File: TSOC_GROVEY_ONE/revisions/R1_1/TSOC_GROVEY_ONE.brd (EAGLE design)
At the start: 44.5 x 30.5 mm, 53 parts, among them J3 NO, J4 6p-2.54, U1 MIC5219 3.3V, U2 ATMEGA328, X1 16MHZ

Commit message: update to Rev 2.0
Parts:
- R10, R4, R5, R7, R8, R9: value 1K 1/10W -> 1K
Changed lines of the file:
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@@
 <setting verticaltext="up"/>
 </settings>
-<grid distance="10" unitdist="mil" unit="mil" style="lines" multiple="1" display="yes" altdistance="5" altunitdist="mil" altunit="mil"/>
+<grid distance="10" unitdist="mil" unit="mm" style="lines" multiple="1" display="yes" altdistance="5" altunitdist="mil" altunit="mil"/>
 <layers>
 <layer number="1" name="Top" color="4" fill="1" visible="yes" active="yes"/>
@@
 <layer number="23" name="tOrigins" color="15" fill="1" visible="yes" active="yes"/>
 <layer number="24" name="bOrigins" color="15" fill="1" visible="yes" active="yes"/>
-<layer number="25" name="tNames" color="7" fill="1" visible="no" active="yes"/>
+<layer number="25" name="tNames" color="7" fill="1" visible="yes" active="yes"/>
 <layer number="26" name="bNames" color="7" fill="1" visible="yes" active="yes"/>
 <layer number="27" name="tValues" color="7" fill="1" visible="no" active="yes"/>
@@
 <layer number="220" name="220bmp" color="21" fill="1" visible="no" active="no"/>
 <layer number="221" name="221bmp" color="22" fill="1" visible="no" active="no"/>
-<layer number="222" name="222bmp" color="23" fill="1" visible="no" active="no"/>
 <layer number="223" name="223bmp" color="24" fill="1" visible="no" active="no"/>
 <layer number="224" name="224bmp" color="25" fill="1" visible="no" active="no"/>
@@
 <attribute name="VALUE" x="42.926" y="24.257" size="0.889" layer="27" font="vector" ratio="11" rot="R270"/>
 </element>
-<element name="R9" library="Seeed-Resistor-2016" package="R0603" value="1K 1/10W" x="34.29" y="20.574" smashed="yes">
+<element name="R9" library="Seeed-Resistor-2016" package="R0603" value="1K" x="34.29" y="20.574" smashed="yes">
 <attribute name="NAME" x="33.528" y="19.939" size="0.8128" layer="25" font="vector" ratio="15" rot="R90"/>
-<attribute name="VALUE" value="1K 1/10W" x="33.274" y="19.431" size="0.4064" layer="27" font="vector"/>
-<attribute name="MPN" value="RC0603JR-071KL" x="34.29" y="20.574" size="1.778" layer="27" display="off"/>
-</element>
-<element name="R10" library="Seeed-Resistor-2016" package="R0603" value="1K 1/10W" x="34.29" y="23.622" smashed="yes" rot="R180">
+<attribute name="VALUE" value="2.2K" x="33.274" y="19.431" size="0.4064" layer="27" font="vector"/>
+<attribute name="MPN" value="RC0603JR-072K2L" x="34.29" y="20.574" size="1.778" layer="27" display="off"/>
+</element>
+<element name="R10" library="Seeed-Resistor-2016" package="R0603" value="1K" x="34.29" y="23.622" smashed="yes" rot="R180">
 <attribute name="NAME" x="32.766" y="24.257" size="0.8128" layer="25" font="vector" ratio="15" rot="R270"/>
-<attribute name="VALUE" value="1K 1/10W" x="35.306" y="24.765" size="0.4064" layer="27" font="vector" rot="R180"/>
-<attribute name="MPN" value="RC0603JR-071KL" x="34.29" y="23.622" size="1.778" layer="27" rot="R180" display="off"/>
-</element>
-<element name="R7" library="Seeed-Resistor-2016" package="R0603" value="1K 1/10W" x="34.29" y="10.16" smashed="yes">
+<attribute name="VALUE" value="2.2K" x="35.306" y="24.765" size="0.4064" layer="27" font="vector" rot="R180"/>
+<attribute name="MPN" value="RC0603JR-072K2L" x="34.29" y="23.622" size="1.778" layer="27" rot="R180" display="off"/>
+</element>
+<element name="R7" library="Seeed-Resistor-2016" package="R0603" value="1K" x="34.29" y="10.16" smashed="yes">
 <attribute name="NAME" x="33.528" y="9.525" size="0.8128" layer="25" font="vector" ratio="15" rot="R90"/>
-<attribute name="VALUE" value="1K 1/10W" x="33.274" y="9.017" size="0.4064" layer="27" font="vector"/>
-<attribute name="MPN" value="RC0603JR-071KL" x="34.29" y="10.16" size="1.778" layer="27" display="off"/>
-</element>
-<element name="R8" library="Seeed-Resistor-2016" package="R0603" value="1K 1/10W" x="34.29" y="13.208" smashed="yes" rot="R180">
+<attribute name="VALUE" value="2.2K" x="33.274" y="9.017" size="0.4064" layer="27" font="vector"/>
+<attribute name="MPN" value="RC0603JR-072K2L" x="34.29" y="10.16" size="1.778" layer="27" display="off"/>
+</element>
+<element name="R8" library="Seeed-Resistor-2016" package="R0603" value="1K" x="34.29" y="13.208" smashed="yes" rot="R180">
 <attribute name="NAME" x="33.528" y="12.573" size="0.8128" layer="25" font="vector" ratio="15" rot="R90"/>
-<attribute name="VALUE" value="1K 1/10W" x="35.306" y="14.351" size="0.4064" layer="27" font="vector" rot="R180"/>
-<attribute name="MPN" value="RC0603JR-071KL" x="34.29" y="13.208" size="1.778" layer="27" rot="R180" display="off"/>
+<attribute name="VALUE" value="2.2K" x="35.306" y="14.351" size="0.4064" layer="27" font="vector" rot="R180"/>
+<attribute name="MPN" value="RC0603JR-072K2L" x="34.29" y="13.208" size="1.778" layer="27" rot="R180" display="off"/>
 </element>
 <element name="R3" library="Seeed-Resistor-2016" package="R0603" value="2.2K" x="9.906" y="9.906" smashed="yes" rot="R180">
@@
 <attribute name="MPN" value="RC0603JR-072K2L" x="9.906" y="6.858" size="1.778" layer="27" display="off"/>
 </element>
-<element name="R5" library="Seeed-Resistor-2016" package="R0603" value="1K 1/10W" x="9.906" y="21.082" smashed="yes">
+<element name="R5" library="Seeed-Resistor-2016" package="R0603" value="1K" x="9.906" y="21.082" smashed="yes">
 <attribute name="NAME" x="10.668" y="21.717" size="0.8128" layer="25" font="vector" ratio="15" rot="R270"/>
-<attribute name="VALUE" value="1K 1/10W" x="8.89" y="19.939" size="0.4064" layer="27" font="vector"/>
-<attribute name="MPN" value="RC0603JR-071KL" x="9.906" y="21.082" size="1.778" layer="27" display="off"/>
-</element>
-<element name="R4" library="Seeed-Resistor-2016" package="R0603" value="1K 1/10W" x="9.906" y="18.034" smashed="yes" rot="R180">
+<attribute name="VALUE" value="2.2K" x="8.89" y="19.939" size="0.4064" layer="27" font="vector"/>
+<attribute name="MPN" value="RC0603JR-072K2L" x="9.906" y="21.082" size="1.778" layer="27" display="off"/>
+</element>
+<element name="R4" library="Seeed-Resistor-2016" package="R0603" value="1K" x="9.906" y="18.034" smashed="yes" rot="R180">
 <attribute name="NAME" x="10.668" y="18.923" size="0.8128" layer="25" font="vector" ratio="15" rot="R270"/>
-<attribute name="VALUE" value="1K 1/10W" x="10.922" y="19.177" size="0.4064" layer="27" font="vector" rot="R180"/>
-<attribute name="MPN" value="RC0603JR-071KL" x="9.906" y="18.034" size="1.778" layer="27" rot="R180" display="off"/>
+<attribute name="VALUE" value="2.2K" x="10.922" y="19.177" size="0.4064" layer="27" font="vector" rot="R180"/>
+<attribute name="MPN" value="RC0603JR-072K2L" x="9.906" y="18.034" size="1.778" layer="27" rot="R180" display="off"/>
 </element>
 <element name="FID4" library="TSOC-ESP8266-BASE" package="MICRO-FIDUCIAL" value="FIDUCIALUFIDUCIAL" x="40.64" y="2.032"/>

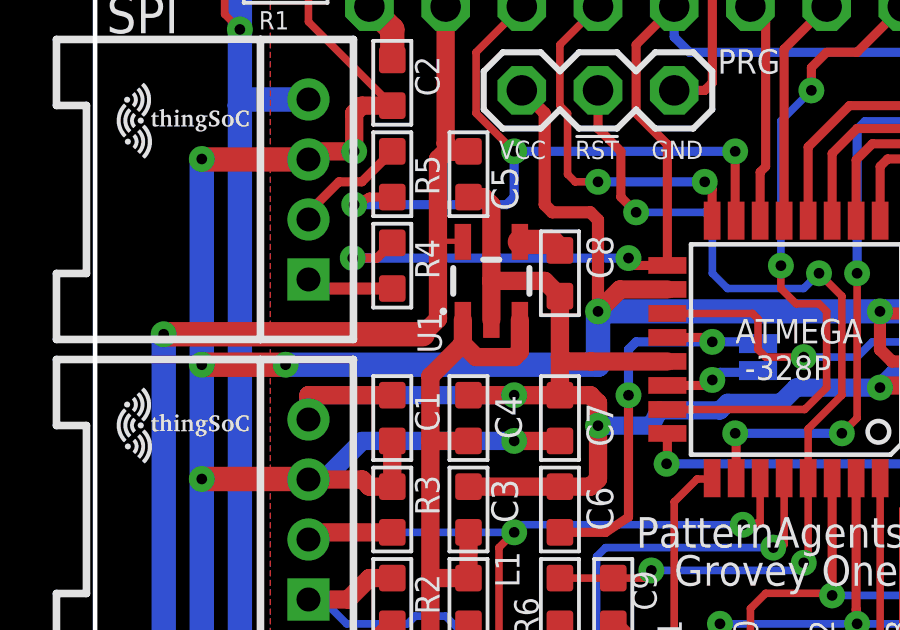
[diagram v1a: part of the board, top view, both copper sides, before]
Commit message: update to Rev 2.0
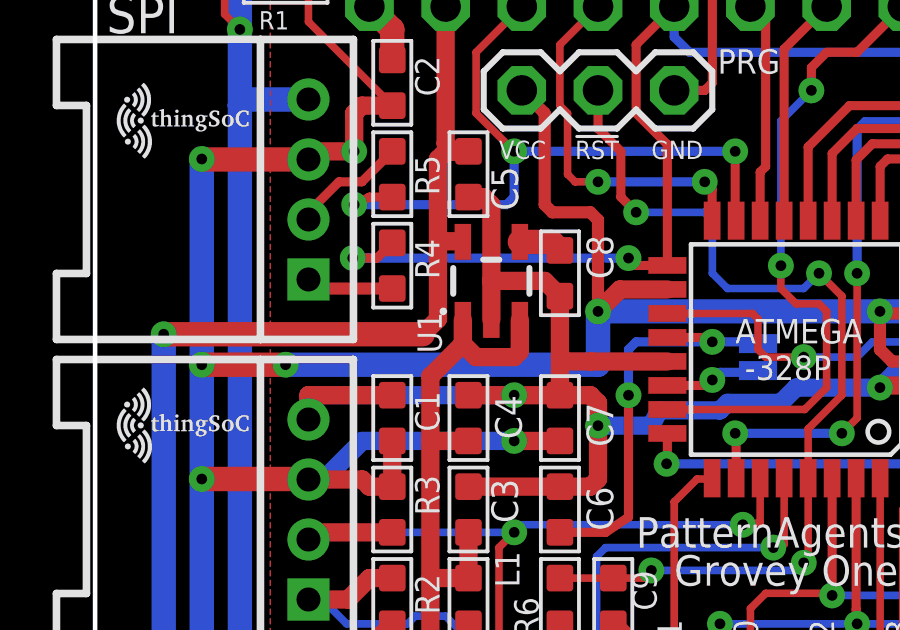
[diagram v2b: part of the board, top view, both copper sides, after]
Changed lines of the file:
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@@
 <wire x1="22.86" y1="13.462" x2="23.368" y2="13.97" width="0.6096" layer="16"/>
 <wire x1="23.368" y1="13.97" x2="26.162" y2="13.97" width="0.6096" layer="16"/>
-<wire x1="12.446" y1="13.8684" x2="12.446" y2="13.81126875" width="0.1778" layer="1"/>
 <wire x1="12.446" y1="13.6906" x2="12.446" y2="13.716" width="0.1778" layer="1"/>
-<wire x1="12.446" y1="13.716" x2="12.446" y2="13.81126875" width="0.1778" layer="1"/>
+<wire x1="12.446" y1="13.716" x2="12.446" y2="13.8684" width="0.1778" layer="1"/>
 <wire x1="12.6238" y1="13.8684" x2="12.446" y2="13.716" width="0.1778" layer="1"/>
 <wire x1="12.6238" y1="13.8684" x2="12.54125" y2="13.81126875" width="0.1778" layer="1"/>
@@
 <wire x1="2.286" y1="15.748" x2="2.286" y2="4.318" width="0.8128" layer="16"/>
 <wire x1="2.286" y1="4.318" x2="5.334" y2="1.27" width="0.8128" layer="16"/>
-<wire x1="11.43" y1="18.8468" x2="12.0904" y2="18.8468" width="0.1778" layer="1"/>
+<wire x1="11.43" y1="18.8468" x2="12.0904" y2="18.8468" width="0.6096" layer="1"/>
 <wire x1="12.0904" y1="18.8468" x2="12.258" y2="18.8261" width="0.1778" layer="1"/>
 <contactref element="TSOC" pad="11B"/>

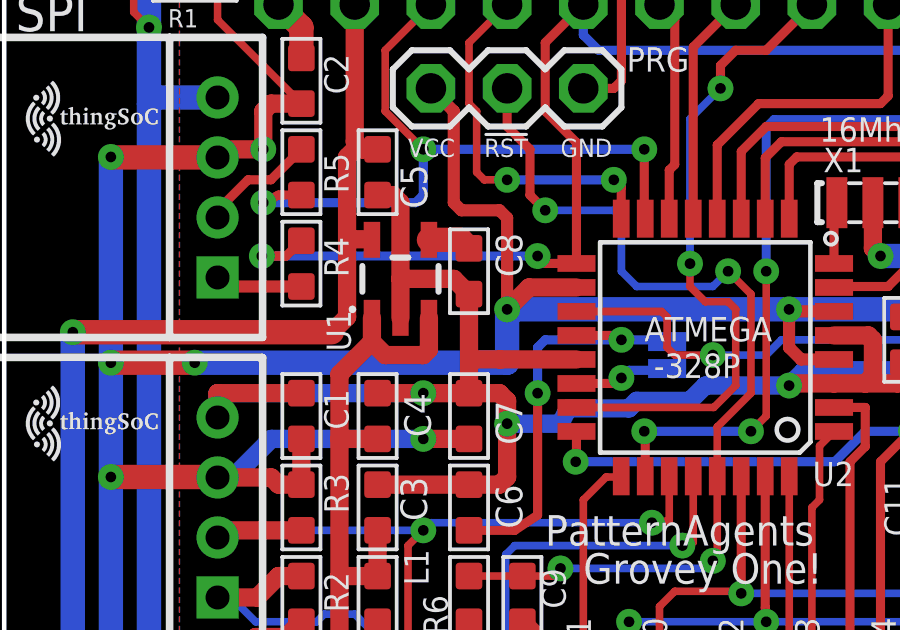
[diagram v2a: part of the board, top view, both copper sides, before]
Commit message: update documetation
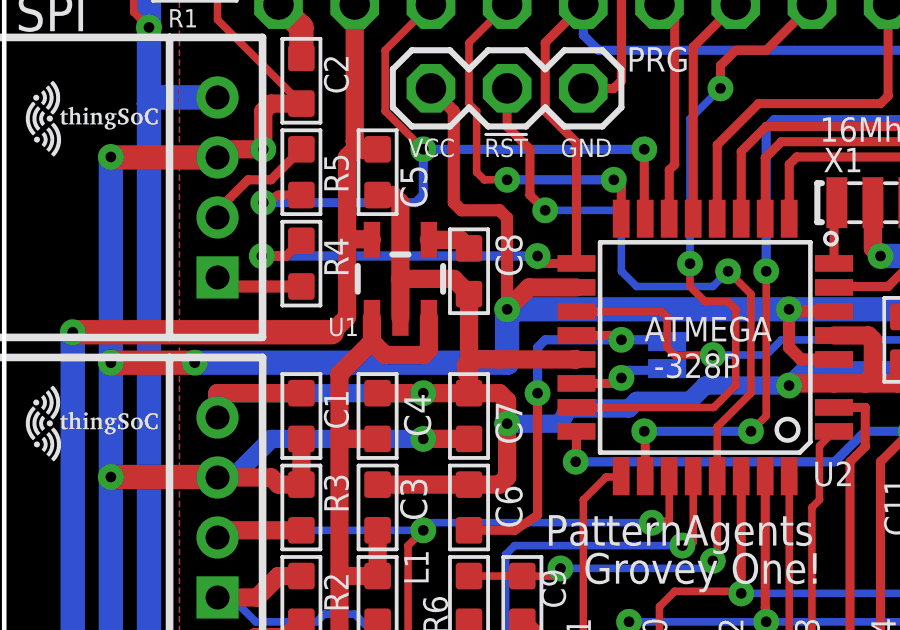
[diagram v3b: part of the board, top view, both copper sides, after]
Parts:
- U1: value MIC5219 3.3V -> AP2112K-3.3V; device TSOC-ESP8266-BASE:SOT23-5 -> SparkFun-PowerIC:SOT23-5
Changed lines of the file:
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@@
 <setting verticaltext="up"/>
 </settings>
-<grid distance="10" unitdist="mil" unit="mm" style="lines" multiple="1" display="yes" altdistance="5" altunitdist="mil" altunit="mil"/>
+<grid distance="10" unitdist="mil" unit="mil" style="lines" multiple="1" display="yes" altdistance="5" altunitdist="mil" altunit="mil"/>
 <layers>
 <layer number="1" name="Top" color="4" fill="1" visible="yes" active="yes"/>
@@
 <layer number="220" name="220bmp" color="21" fill="1" visible="no" active="no"/>
 <layer number="221" name="221bmp" color="22" fill="1" visible="no" active="no"/>
+<layer number="222" name="222bmp" color="23" fill="1" visible="no" active="no"/>
 <layer number="223" name="223bmp" color="24" fill="1" visible="no" active="no"/>
 <layer number="224" name="224bmp" color="25" fill="1" visible="no" active="no"/>
@@
 <attribute name="NAME" x="21.844" y="0.635" size="0.635" layer="33" ratio="10"/>
 </element>
-<element name="U1" library="TSOC-ESP8266-BASE" package="SOT23-5" value="MIC5219 3.3V" x="13.208" y="17.526" smashed="yes">
-<attribute name="PROD_ID" value="VREG-09872" x="9.906" y="28.956" size="1.778" layer="27" display="off"/>
-<attribute name="NAME" x="11.557" y="15.113" size="0.8128" layer="25" font="vector" ratio="15" rot="R90"/>
-<attribute name="VALUE" x="12.2555" y="17.3355" size="0.4064" layer="27"/>
-</element>
 <element name="C8" library="Seeed-Capacitor-2016" package="C0603" value="470Pf" x="15.494" y="17.78" smashed="yes">
 <attribute name="MPN" value="CC0603KRX7R9BB104" x="7.874" y="34.544" size="1.778" layer="27" display="off"/>
@@
 <attribute name="VALUE" x="11.684" y="-1.905" size="1.27" layer="27"/>
 </element>
+<element name="U1" library="SparkFun-PowerIC" package="SOT23-5" value="AP2112K-3.3V" x="13.208" y="17.526" smashed="yes">
+<attribute name="PROD_ID" value="VREG-12457" x="9.906" y="22.352" size="1.778" layer="27" display="off"/>
+<attribute name="NAME" x="10.795" y="15.621" size="0.6096" layer="25" font="vector" ratio="15"/>
+<attribute name="VALUE" x="12.2555" y="17.3355" size="0.4064" layer="27"/>
+</element>
 </elements>
 <signals>
 <signal name="5V0">
 <contactref element="L1" pad="1"/>
-<contactref element="U1" pad="1"/>
 <contactref element="C4" pad="1"/>
-<contactref element="U1" pad="3"/>
 <contactref element="J3" pad="3"/>
 <contactref element="C3" pad="2"/>
@@
 <wire x1="10.414" y1="1.27" x2="10.414" y2="3.048" width="0.6096" layer="16"/>
 <wire x1="12.446" y1="7.62" x2="12.446" y2="9.144" width="0.6096" layer="1"/>
-<wire x1="14.158" y1="16.2259" x2="14.158" y2="15.174" width="0.6096" layer="1"/>
 <wire x1="14.158" y1="15.174" x2="13.97" y2="14.986" width="0.6096" layer="1"/>
 <wire x1="13.97" y1="14.986" x2="12.7" y2="14.986" width="0.6096" layer="1"/>
 <wire x1="12.7" y1="14.986" x2="12.258" y2="15.428" width="0.6096" layer="1"/>
-<wire x1="12.258" y1="16.2259" x2="12.258" y2="15.428" width="0.6096" layer="1"/>
 <wire x1="11.176" y1="14.346" x2="11.176" y2="12.192" width="0.6096" layer="1"/>
 <wire x1="11.176" y1="12.192" x2="11.176" y2="7.62" width="0.6096" layer="1"/>
@@
 <wire x1="10.414" y1="4.572" x2="11.176" y2="5.334" width="0.6096" layer="16"/>
 <wire x1="12.446" y1="7.62" x2="11.176" y2="7.62" width="0.6096" layer="1"/>
+<contactref element="U1" pad="3"/>
+<contactref element="U1" pad="1"/>
+<wire x1="12.258" y1="16.2259" x2="12.258" y2="15.428" width="0.6096" layer="1"/>
+<wire x1="14.158" y1="15.174" x2="14.158" y2="16.2259" width="0.6096" layer="1"/>
 </signal>
 <signal name="GND">
@@
 <contactref element="TSOC" pad="12C"/>
 <contactref element="C8" pad="2"/>
-<contactref element="U1" pad="2"/>
 <contactref element="C4" pad="2"/>
 <contactref element="J4" pad="1"/>
@@
 <wire x1="9.906" y1="25.908" x2="9.144" y2="26.67" width="0.8128" layer="1"/>
 <wire x1="13.208" y1="20.066" x2="13.208" y2="17.526" width="0.6096" layer="1"/>
-<wire x1="13.208" y1="17.526" x2="13.208" y2="16.2259" width="0.6096" layer="1"/>
 <wire x1="9.906" y1="13.716" x2="7.112" y2="13.716" width="0.6096" layer="1"/>
 <wire x1="9.144" y1="26.67" x2="9.144" y2="28.448" width="0.8128" layer="16"/>
@@
 <wire x1="14.986" y1="17.526" x2="13.208" y2="17.526" width="0.6096" layer="1"/>
 <wire x1="15.494" y1="17.018" x2="15.494" y2="14.986" width="0.6096" layer="1"/>
-<wire x1="15.494" y1="14.986" x2="15.494" y2="13.716" width="0.6096" layer="1"/>
+<wire x1="15.494" y1="14.986" x2="15.494" y2="14.732" width="0.6096" layer="1"/>
+<wire x1="15.494" y1="14.732" x2="15.494" y2="13.716" width="0.6096" layer="1"/>
 <wire x1="19.0754" y1="14.84" x2="16.5354" y2="14.84" width="0.6096" layer="1"/>
 <wire x1="16.5354" y1="14.84" x2="15.64" y2="14.84" width="0.6096" layer="1"/>
-<wire x1="15.64" y1="14.84" x2="15.494" y2="14.986" width="0.6096" layer="1"/>
 <wire x1="12.446" y1="13.716" x2="13.97" y2="13.716" width="0.6096" layer="1"/>
 <wire x1="13.97" y1="13.716" x2="15.494" y2="13.716" width="0.6096" layer="1"/>
@@
 <wire x1="12.6238" y1="13.8684" x2="12.446" y2="13.716" width="0.1778" layer="1"/>
 <wire x1="12.6238" y1="13.8684" x2="12.54125" y2="13.81126875" width="0.1778" layer="1"/>
+<contactref element="U1" pad="2"/>
+<wire x1="13.208" y1="16.2259" x2="13.208" y2="17.526" width="0.6096" layer="1"/>
+<wire x1="15.64" y1="14.84" x2="15.494" y2="14.986" width="0.6096" layer="1"/>
+<wire x1="19.0754" y1="14.84" x2="19.0373" y2="14.84" width="0.6096" layer="1"/>
+<wire x1="19.0373" y1="14.84" x2="19.0246" y2="14.8527" width="0.6096" layer="1"/>
+<wire x1="15.39874375" y1="14.4018" x2="15.39874375" y2="14.63674375" width="0.6096" layer="1"/>
+<wire x1="15.39874375" y1="14.63674375" x2="15.494" y2="14.732" width="0.6096" layer="1"/>
+<wire x1="26.162" y1="13.97" x2="26.232" y2="14.04" width="0" layer="19" extent="1-1"/>
+<wire x1="15.58926875" y1="10.76325" x2="15.494" y2="10.668" width="0" layer="19" extent="1-1"/>
 </signal>
 <signal name="3V3">
-<contactref element="U1" pad="5"/>
 <contactref element="J3" pad="1"/>
 <contactref element="C5" pad="2"/>
@@
 <wire x1="2.286" y1="4.318" x2="5.334" y2="1.27" width="0.8128" layer="16"/>
 <wire x1="11.43" y1="18.8468" x2="12.0904" y2="18.8468" width="0.6096" layer="1"/>
-<wire x1="12.0904" y1="18.8468" x2="12.258" y2="18.8261" width="0.1778" layer="1"/>
 <contactref element="TSOC" pad="11B"/>
 <wire x1="11.684" y1="26.67" x2="11.684" y2="22.098" width="0.6096" layer="1"/>
 <wire x1="11.684" y1="22.098" x2="11.938" y2="21.844" width="0.6096" layer="1"/>
+<contactref element="U1" pad="5"/>
+<wire x1="12.258" y1="18.8261" x2="12.1111" y2="18.8261" width="0.6096" layer="1"/>
+<wire x1="12.1111" y1="18.8261" x2="12.0904" y2="18.8468" width="0.6096" layer="1"/>
 </signal>
 <signal name="VCC">
@@
 </signal>
 <signal name="BYPASS1">
+<contactref element="C8" pad="1"/>
+<wire x1="15.2099" y1="18.8261" x2="15.494" y2="18.542" width="0.6096" layer="1"/>
 <contactref element="U1" pad="4"/>
-<contactref element="C8" pad="1"/>
-<wire x1="14.158" y1="18.8261" x2="15.2099" y2="18.8261" width="0.8128" layer="1"/>
-<wire x1="15.2099" y1="18.8261" x2="15.494" y2="18.542" width="0.8128" layer="1"/>
+<wire x1="14.158" y1="18.8261" x2="15.2099" y2="18.8261" width="0.6096" layer="1"/>
 </signal>
 <signal name="A7">
